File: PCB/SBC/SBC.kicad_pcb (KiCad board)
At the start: 2 copper layers, 127 x 101.6 mm, 78 parts, among them J1 ZTO-80 Bus, J10 Conn_01x02, J11 CTCHDR, J12 Conn_01x02, J2 5V_IN, J3 DB9_Male_MountingHoles, J4 CPUHDR, J5 PIOHDR, J6 PIOHDR, J7 SIOHDR, J8 SIOHDR, J9 Conn_01x02, SW1 Reset, U1 Z80CPU, U10 74HC138, U2 Z80SIO0, U3 MAX202, U4 28C256, U5 Z80PIO, U6 AS6C62256, U7 Z80CTC, U8 74HC139, U9 ULN2803A, X1 SYS_CLK, X2 1.8432MHz

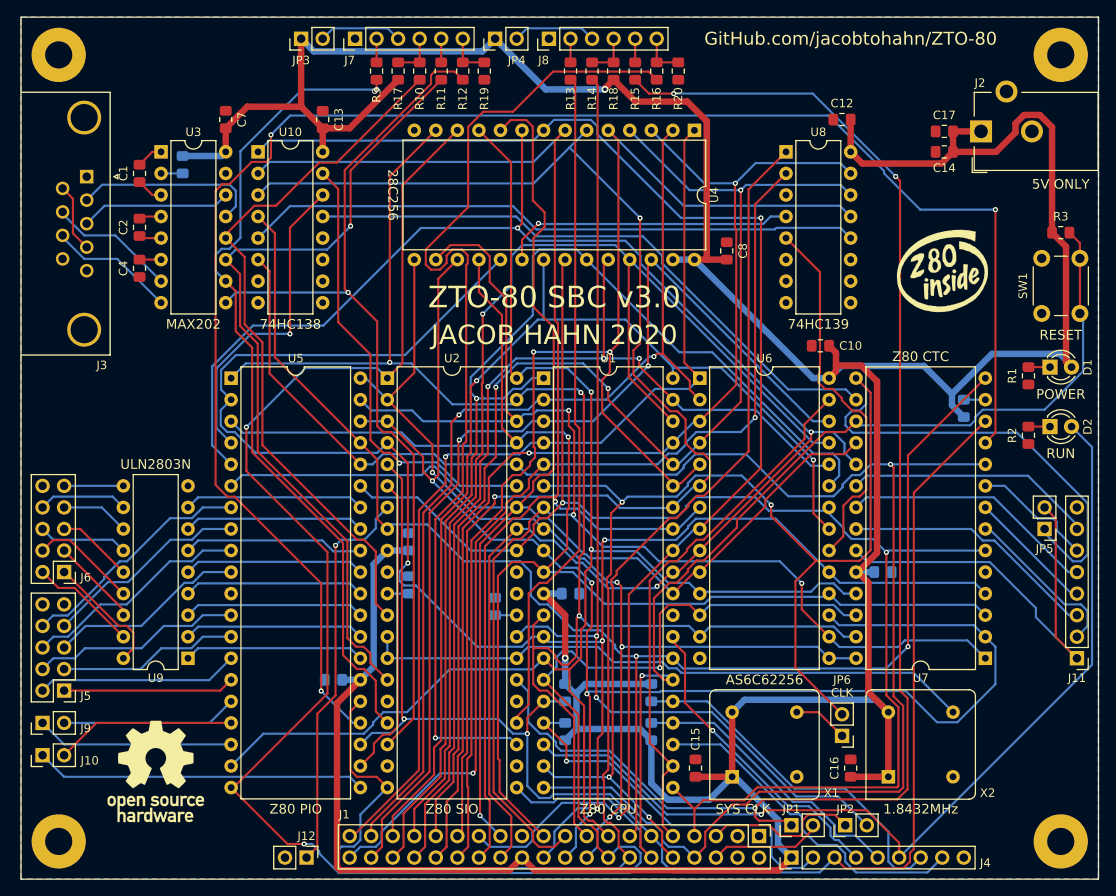
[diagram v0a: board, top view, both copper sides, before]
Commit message: Updated SBC to v3.1
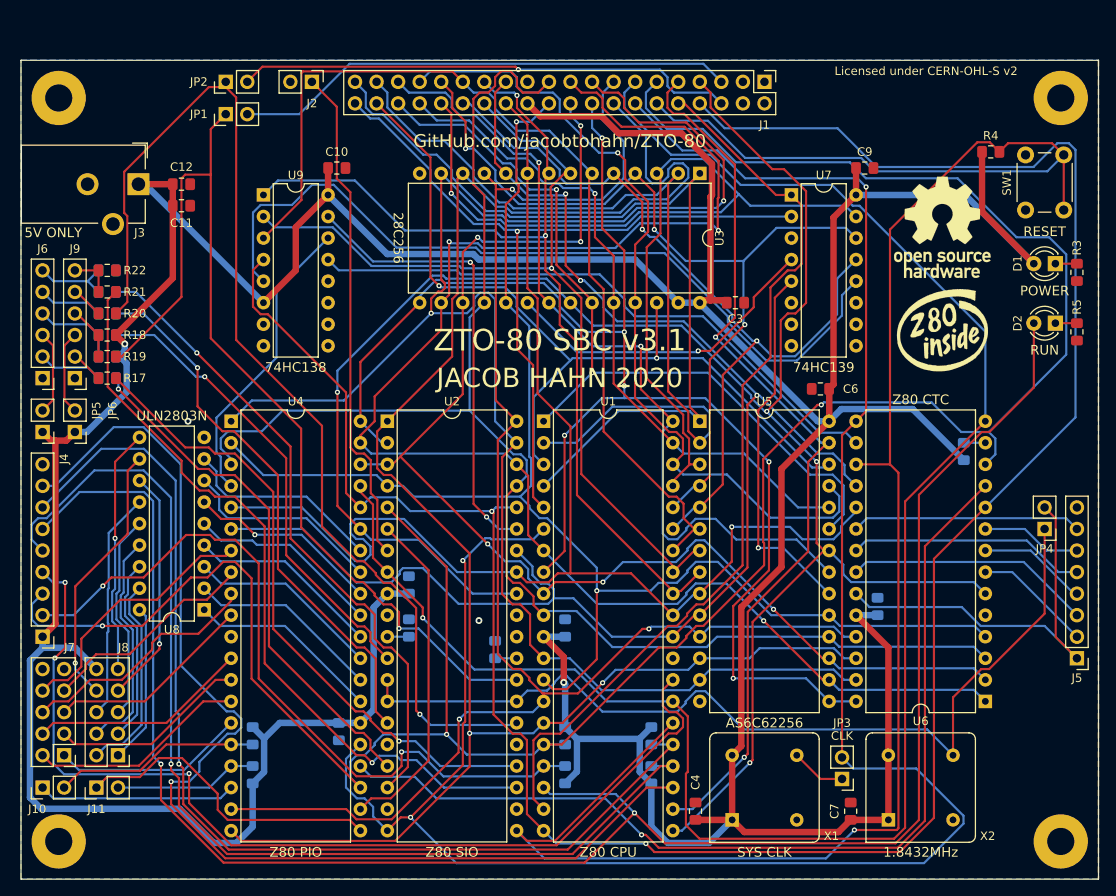
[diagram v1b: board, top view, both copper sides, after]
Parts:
- removed C13, C14, C15, C16: 0.1u, Capacitor_SMD:C_0805_2012Metric_Pad1.15x1.40mm_HandSolder
- removed C17: 10u, Capacitor_SMD:C_0805_2012Metric_Pad1.15x1.40mm_HandSolder
- removed J12: Conn_01x02, Connector_PinHeader_2.54mm:PinHeader_1x02_P2.54mm_Vertical
- removed the J5 at (87.6, 130.8)
- removed the J6 at (87.6, 116.8)
- removed the J9 at (85.1, 134.6)
- removed the JP6 at (179.3, 136.1)
- removed the R21 at (128.3, 118.4)
- removed the R22 at (138.4, 120.9)
- removed the R6 at (156.8, 131.1)
- removed the R7 at (156.8, 135.6)
- removed the R8 at (193.7, 97.5)
- removed U10: 74HC138, Package_DIP:DIP-16_W7.62mm
- added J11: Conn_01x02, Connector_PinHeader_2.54mm:PinHeader_1x02_P2.54mm_Vertical, F.Cu at (91.4, 142.2)
- added J7: PIOHDR, Connector_PinHeader_2.54mm:PinHeader_2x05_P2.54mm_Vertical, F.Cu at (87.6, 138.4)
- added J8: PIOHDR, Connector_PinHeader_2.54mm:PinHeader_2x05_P2.54mm_Vertical, F.Cu at (94.0, 138.4)
- added JP3: Jumper_2_Open, Connector_PinHeader_2.54mm:PinHeader_1x02_P2.54mm_Vertical, F.Cu at (179.3, 141.2)
- added R11: 10k, Resistor_SMD:R_0805_2012Metric_Pad1.15x1.40mm_HandSolder, B.Cu at (146.7, 136.1)
- added R12: 10k, Resistor_SMD:R_0805_2012Metric_Pad1.15x1.40mm_HandSolder, B.Cu at (146.7, 140.7)
- added R13: 10k, Resistor_SMD:R_0805_2012Metric_Pad1.15x1.40mm_HandSolder, B.Cu at (156.8, 136.1)
- added R14: 10k, Resistor_SMD:R_0805_2012Metric_Pad1.15x1.40mm_HandSolder, B.Cu at (156.8, 140.7)
- added R15: 10k, Resistor_SMD:R_0805_2012Metric_Pad1.15x1.40mm_HandSolder, B.Cu at (193.7, 102.6)
- added R23: 10k, Resistor_SMD:R_0805_2012Metric_Pad1.15x1.40mm_HandSolder, B.Cu at (109.9, 136.1)
- added R24: 10k, Resistor_SMD:R_0805_2012Metric_Pad1.15x1.40mm_HandSolder, B.Cu at (109.9, 140.7)
- C1, C2, C8: moved to B.Cu
- C11, C3, C6, C9: moved to F.Cu
- C12: value 0.1u -> 10u
- J2: value 5V_IN -> Conn_01x02; footprint BarrelJack:BarrelJack_CUI_PJ-102A_Horizontal -> Connector_PinHeader_2.54mm:PinHeader_1x02_P2.54mm_Vertical
- J3: value DB9_Male_MountingHoles -> 5V_IN; footprint Connector_Dsub:DSUB-9_Male_Horizontal_P2.77x2.84mm_EdgePinOffset4.94mm_Housed_MountingHolesOffset7.48mm -> BarrelJack:BarrelJack_CUI_PJ-102A_Horizontal
- R1, R2: value 220 -> 10k; moved to B.Cu
- R10: renamed from R12; moved to B.Cu
- R16: renamed from R19; moved to B.Cu
- R3: value 1k -> 220
- R4: value 1k -> 10k; moved to F.Cu
- R5: value 1k -> 220; moved to F.Cu
- R6: renamed from R9; moved to B.Cu
- R7: renamed from R17; moved to B.Cu
- R8: renamed from R10; moved to B.Cu
- R9: renamed from R11; moved to B.Cu
- U3: value MAX202 -> 28C256; footprint Package_DIP:DIP-16_W7.62mm -> Package_DIP:DIP-28_W15.24mm
- U4: value 28C256 -> Z80PIO; footprint Package_DIP:DIP-28_W15.24mm -> Package_DIP:DIP-40_W15.24mm
- U5: value Z80PIO -> AS6C62256; footprint Package_DIP:DIP-40_W15.24mm -> Package_DIP:DIP-28_W15.24mm
- U6: value AS6C62256 -> Z80CTC
- U7: value Z80CTC -> 74HC139; footprint Package_DIP:DIP-28_W15.24mm -> Package_DIP:DIP-16_W7.62mm
- U8: value 74HC139 -> ULN2803A; footprint Package_DIP:DIP-16_W7.62mm -> Package_DIP:DIP-18_W7.62mm
- U9: value ULN2803A -> 74HC138; footprint Package_DIP:DIP-18_W7.62mm -> Package_DIP:DIP-16_W7.62mm
- moved JP2 114.1 mm to (106.7, 59.1)
- moved REF** 112.7 mm to (191.1, 76.2)
- moved C7 109.9 mm to (180.3, 145.0)
- moved JP1 107.1 mm to (106.7, 62.9)
- moved C11 93.3 mm to (101.5, 73.7)
- moved J4 92.0 mm to (85.1, 124.5), turned to 180 degrees
- moved C4 91.6 mm to (162.1, 145.0), turned to 90 degrees
- moved J1 88.9 mm to (170.2, 59.1)
- moved U8 87.3 mm to (104.1, 121.3), turned to 180 degrees
- moved C9 87.0 mm to (182.0, 69.2), turned to 0 degrees
- moved R4 81.1 mm to (196.8, 67.3), turned to 180 degrees
- moved J2 79.1 mm to (116.8, 59.1), turned to 270 degrees
- moved R1 78.8 mm to (128.3, 123.4), turned to 270 degrees
- moved C12 78.2 mm to (101.5, 71.1), turned to 0 degrees
- moved R5 76.5 mm to (207.0, 88.5)
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- renumbered J11 to J5, J7 to J6, J8 to J9, JP5 to JP4, JP3 to JP5, JP4 to JP6, R13 to R17, R14 to R19, R15 to R20, R16 to R21, R20 to R22
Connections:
- C1 pad 1: Net-(C1-Pad1) -> VCC
- C1 pad 2: Net-(C1-Pad2) -> GND
- C2 pad 1: Net-(C2-Pad1) -> VCC
- C2 pad 2: Net-(C2-Pad2) -> GND
- C3 pad 1: Net-(C3-Pad1) -> VCC
- C3 pad 2: VCC -> GND
- C4 pad 1: Net-(C4-Pad1) -> VCC
- J10 pad 1: /BRDY -> /ARDY
- J10 pad 2: /BSTB -> /ASTB
- J2 pad 1: VCC -> /EXIEI
- J2 pad 2: GND -> Net-(J2-Pad2)
- J3 pad 1: Net-(J3-Pad1) -> VCC
- J3 pad 2: /RX232 -> GND
- J3 pad 3: /TX232 -> GND
- JP1 pad 1: /TXB -> /RXB
- JP1 pad 2: Net-(J1-Pad6) -> Net-(J1-Pad5)
- JP2 pad 1: Net-(J1-Pad5) -> /TXB
- JP2 pad 2: /RXB -> Net-(J1-Pad6)
- JP4 pad 1: /CLK -> /BCLK
- R1 pad 2: Net-(D1-Pad1) -> Net-(R1-Pad2)
- R2 pad 2: Net-(D2-Pad1) -> Net-(R2-Pad2)
- R3 pad 1: /RST -> GND
- R3 pad 2: VCC -> Net-(D1-Pad1)
- R4 pad 1: VCC -> /RST
- R4 pad 2: /INT -> VCC
- R5 pad 1: VCC -> GND
- R5 pad 2: /NMI -> Net-(D2-Pad1)
- U2 pad 11: Net-(R21-Pad2) -> Net-(R1-Pad2)
- U2 pad 29: Net-(R22-Pad2) -> Net-(R2-Pad2)
- U3 pad 1: Net-(C1-Pad1) -> /A14
- U3 pad 10: /RTSA -> /A0
- U3 pad 11: /TXA -> /D0
- U3 pad 12: /RXA -> /D1
- U3 pad 13: /RX232 -> /D2
- U3 pad 14: /TX232 -> GND
- U3 pad 15: GND -> /D3
- U3 pad 16: VCC -> /D4
- U3 pad 2: Net-(C3-Pad1) -> /A12
- U3 pad 3: Net-(C1-Pad2) -> /A7
- U3 pad 4: Net-(C2-Pad1) -> /A6
- U3 pad 5: Net-(C2-Pad2) -> /A5
- U3 pad 6: Net-(C4-Pad1) -> /A4
- U3 pad 7: /RTS232 -> /A3
- U3 pad 8: /CTS232 -> /A2
- U3 pad 9: /CTSA -> /A1
- U4 pad 1: /A14 -> /D2
- U4 pad 10: /A0 -> /PA4
- U4 pad 11: /D0 -> GND
- U4 pad 12: /D1 -> /PA3
- U4 pad 13: /D2 -> /PA2
- U4 pad 14: GND -> /PA1
- U4 pad 15: /D3 -> /PA0
- U4 pad 16: /D4 -> /ASTB
- U4 pad 17: /D5 -> /BSTB
- U4 pad 18: /D6 -> /ARDY
- U4 pad 19: /D7 -> /D0
- U4 pad 2: /A12 -> /D7
- U4 pad 20: /ROMCE -> /D1
- U4 pad 21: /A10 -> /BRDY
- U4 pad 22: /RD -> /SIOIEI
- U4 pad 23: /A11 -> /INT
- U4 pad 24: /A9 -> /PIOIEI
- U4 pad 25: /A8 -> /CLK
- U4 pad 26: /A13 -> VCC
- U4 pad 27: VCC -> /DB0
- U4 pad 28: VCC -> /DB1
- U4 pad 3: /A7 -> /D6
- U4 pad 4: /A6 -> /PIOCE
- U4 pad 5: /A5 -> /A1
- U4 pad 6: /A4 -> /A0
- U4 pad 7: /A3 -> /PA7
- U4 pad 8: /A2 -> /PA6
- U4 pad 9: /A1 -> /PA5
- U5 pad 1: /D2 -> /A14
- U5 pad 10: /PA4 -> /A0
- U5 pad 11: GND -> /D0
- U5 pad 12: /PA3 -> /D1
- U5 pad 13: /PA2 -> /D2
- U5 pad 14: /PA1 -> GND
- U5 pad 15: /PA0 -> /D3
- U5 pad 16: /ASTB -> /D4
- U5 pad 17: /BSTB -> /D5
- U5 pad 18: /ARDY -> /D6
- U5 pad 19: /D0 -> /D7
- U5 pad 2: /D7 -> /A12
- U5 pad 20: /D1 -> /RAMCE
- U5 pad 21: /BRDY -> /A10
- U5 pad 22: /SIOIEI -> /RD
- U5 pad 23: /INT -> /A11
- U5 pad 24: /PIOIEI -> /A9
- U5 pad 25: /CLK -> /A8
- U5 pad 26: VCC -> /A13
- U5 pad 27: /DB0 -> /WR
- U5 pad 28: /DB1 -> VCC
- U5 pad 3: /D6 -> /A7
- U5 pad 4: /PIOCE -> /A6
- U5 pad 5: /A1 -> /A5
- U5 pad 6: /A0 -> /A4
- U5 pad 7: /PA7 -> /A3
- U5 pad 8: /PA6 -> /A2
- U5 pad 9: /PA5 -> /A1
- U6 pad 1: /A14 -> /D4
- U6 pad 10: /A0 -> /IORQ
- U6 pad 11: /D0 -> /PIOIEI
- U6 pad 12: /D1 -> /INT
- U6 pad 13: /D2 -> /IEI
- U6 pad 14: GND -> /M1
- U6 pad 15: /D3 -> /CLK
- U6 pad 16: /D4 -> /CTCCE
- U6 pad 17: /D5 -> /RST
- U6 pad 18: /D6 -> /A0
- U6 pad 19: /D7 -> /A1
- U6 pad 2: /A12 -> /D5
- U6 pad 20: /RAMCE -> /CT3
- U6 pad 21: /A10 -> /CT2
- U6 pad 22: /RD -> /CT1
- U6 pad 23: /A11 -> /CT0
- U6 pad 24: /A9 -> VCC
- U6 pad 25: /A8 -> /D0
- U6 pad 26: /A13 -> /D1
- U6 pad 27: /WR -> /D2
- U6 pad 28: VCC -> /D3
- U6 pad 3: /A7 -> /D6
- U6 pad 4: /A6 -> /D7
- U6 pad 5: /A5 -> GND
- U6 pad 6: /A4 -> /RD
- U6 pad 7: /A3 -> /ZT0
- U6 pad 8: /A2 -> /ZT1
- U6 pad 9: /A1 -> /ZT2
- U7 pad 1: /D4 -> /MREQ
- U7 pad 10: /IORQ -> Net-(U7-Pad10)
- U7 pad 11: /PIOIEI -> Net-(U7-Pad11)
- U7 pad 12: /INT -> /IOEN
- U7 pad 13: /IEI -> /A5
- U7 pad 14: /M1 -> /A6
- U7 pad 15: /CLK -> /A7
- U7 pad 16: /CTCCE -> VCC
- U7 pad 2: /D5 -> /A15
- U7 pad 3: /D6 -> GND
- U7 pad 4: /D7 -> /ROMCE
- U7 pad 5: GND -> /RAMCE
- U7 pad 6: /RD -> Net-(U7-Pad6)
- U7 pad 7: /ZT0 -> Net-(U7-Pad7)
- U7 pad 8: /ZT1 -> GND
- U7 pad 9: /ZT2 -> Net-(U7-Pad9)
- U8 pad 1: /MREQ -> /DB0
- U8 pad 10: Net-(U8-Pad10) -> /K
- U8 pad 11: Net-(U8-Pad11) -> /PB7
- U8 pad 12: /IOEN -> /PB6
- U8 pad 13: /A5 -> /PB5
- U8 pad 14: /A6 -> /PB4
- U8 pad 15: /A7 -> /PB3
- U8 pad 16: VCC -> /PB2
- U8 pad 2: /A15 -> /DB1
- U8 pad 3: GND -> /DB2
- U8 pad 4: /ROMCE -> /DB3
- U8 pad 5: /RAMCE -> /DB4
- U8 pad 6: Net-(U8-Pad6) -> /DB5
- U8 pad 7: Net-(U8-Pad7) -> /DB6
- U8 pad 8: GND -> /DB7
- U8 pad 9: Net-(U8-Pad9) -> GND
- U9 pad 1: /DB0 -> /A2
- U9 pad 10: /K -> Net-(U9-Pad10)
- U9 pad 11: /PB7 -> Net-(U9-Pad11)
- U9 pad 12: /PB6 -> Net-(U9-Pad12)
- U9 pad 13: /PB5 -> /CTCCE
- U9 pad 14: /PB4 -> /PIOCE
- U9 pad 15: /PB3 -> /SIOCE
- U9 pad 16: /PB2 -> VCC
- U9 pad 2: /DB1 -> /A3
- U9 pad 3: /DB2 -> /A4
- U9 pad 4: /DB3 -> /IORQ
- U9 pad 5: /DB4 -> /IOEN
- U9 pad 6: /DB5 -> VCC
- U9 pad 7: /DB6 -> Net-(U9-Pad7)
- U9 pad 8: /DB7 -> GND
- U9 pad 9: GND -> Net-(U9-Pad9)
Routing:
- net /INT: track 173.8 -> 293.1 mm, vias 2 -> 3
- net /HLT: track 110.1 -> 225.0 mm, vias 1 -> 2
- net /BACK: track 40.1 -> 134.9 mm, vias 0 -> 1
- net /RST: track 137.8 -> 232.3 mm
- net /WAIT: track 33.8 -> 128.1 mm, vias 0 -> 1
- net /PIOIEI: track 200.7 -> 114.3 mm, vias 3 -> 1
- net /BREQ: track 42.5 -> 126.2 mm, vias 0 -> 1
- net /RFSH: track 36.6 -> 118.7 mm, vias 1 -> 3
- net /IORQ: track 198.8 -> 279.2 mm, vias 1 -> 2
- net /A5: track 156.6 -> 96.3 mm
- net VCC: track 512.3 -> 571.3 mm
- net /RD: track 174.1 -> 232.7 mm, vias 2 -> 4
- net /D3: track 122.5 -> 175.2 mm, vias 4 -> 6
- net /A2: track 164.6 -> 112.1 mm
- net /A1: track 207.0 -> 157.9 mm, vias 3 -> 1
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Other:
- board size 127 x 101.6 mm -> 127 x 96.5 mm
- rule trace_min: 0.2 -> 0.254
- board text added: "PIO"
- board text added: "Serial"
- board text added: "ZTO-80 SBC v3.1"
- board text removed: "CTS"
- board text removed: "GND"
- board text removed: "MAX202"
- board text removed: "RTS"
- board text removed: "RX"
- board text removed: "TX"
- board text removed: "VCC"
- board text removed: "VCC A"
- board text removed: "VCC B"
- board text removed: "ZTO-80 SBC v3.0"
